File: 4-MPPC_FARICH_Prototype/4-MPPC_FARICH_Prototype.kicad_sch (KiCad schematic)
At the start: 33 parts, among them J1 1778764, J2 ST4-40-1.00-L-D-P-TR, J3 ST4-40-1.00-L-D-P-TR, J4 ST4-40-1.00-L-D-P-TR, J5 ST4-40-1.00-L-D-P-TR, J6 ST4-40-1.00-L-D-P-TR, J7 ST4-40-1.00-L-D-P-TR, J8 ST4-40-1.00-L-D-P-TR, J9 ST4-40-1.00-L-D-P-TR

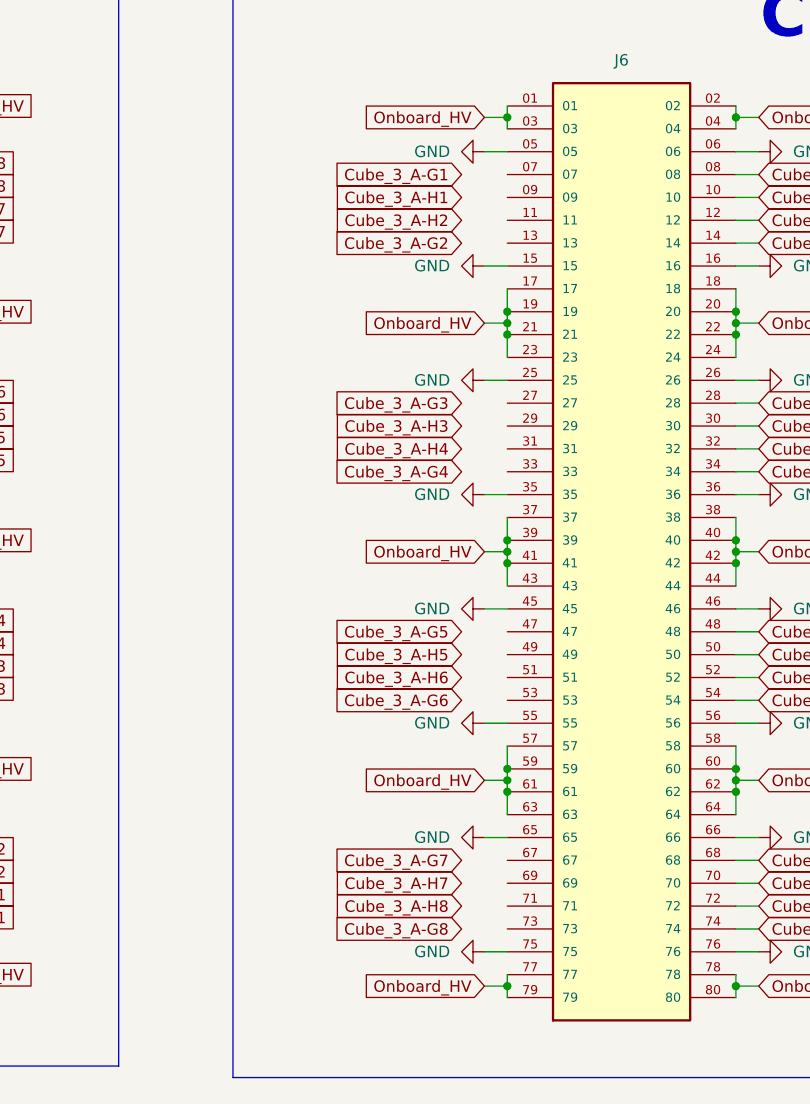
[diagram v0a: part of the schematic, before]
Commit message: .
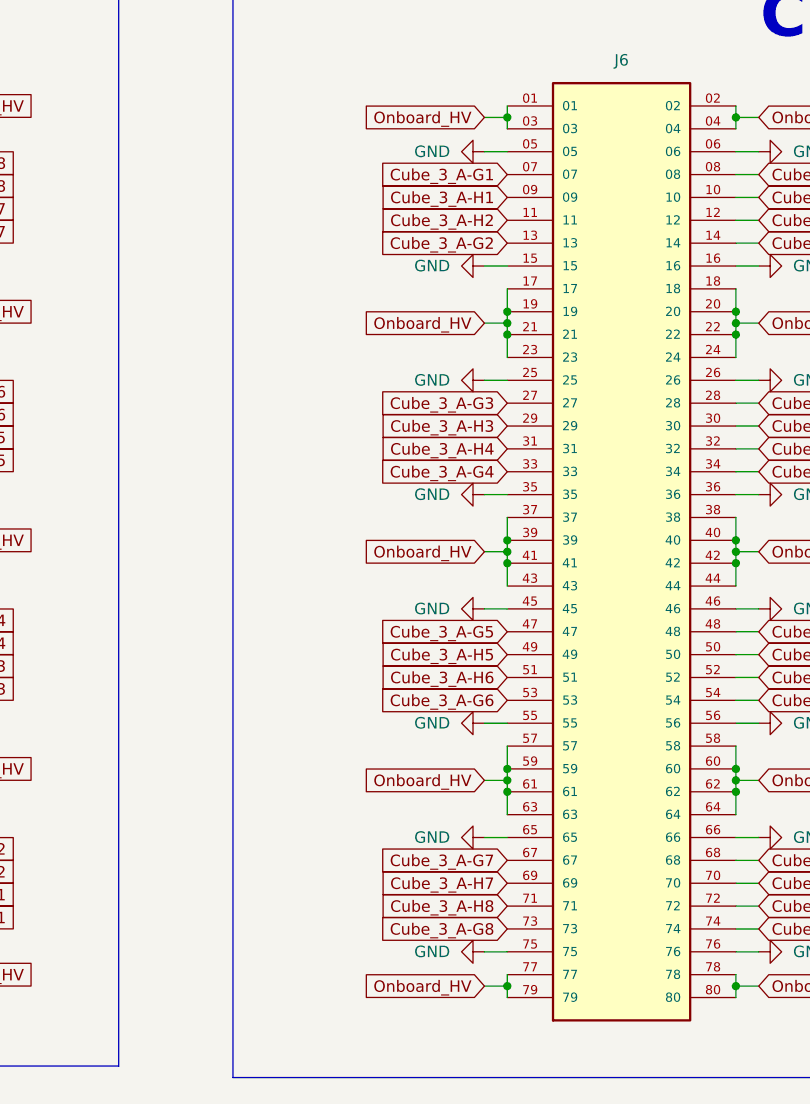
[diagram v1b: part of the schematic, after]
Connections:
- net Cube_3_A-G1: now also J6.07
- net Cube_3_A-G2: now also J6.13
- net Cube_3_A-G3: now also J6.27
- net Cube_3_A-G4: now also J6.33
- net Cube_3_A-G5: now also J6.47
- net Cube_3_A-G6: now also J6.53
- net Cube_3_A-G7: now also J6.67
- net Cube_3_A-G8: now also J6.73
- net Cube_3_A-H1: now also J6.09
- net Cube_3_A-H2: now also J6.11
- net Cube_3_A-H3: now also J6.29
- net Cube_3_A-H4: now also J6.31
- net Cube_3_A-H5: now also J6.49
- net Cube_3_A-H6: now also J6.51
- net Cube_3_A-H7: now also J6.69
- net Cube_3_A-H8: now also J6.71
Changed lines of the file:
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@@
 	(global_label "Cube_3_A-H4"
 		(shape input)
-		(at 232.41 320.04 180)
+		(at 237.49 320.04 180)
 		(fields_autoplaced yes)
 		(effects
@@
 		)
 		(property "Intersheetrefs" "${INTERSHEET_REFS}"
-			(at 216.4225 320.04 0)
+			(at 221.5025 320.04 0)
 			(effects
 				(font
@@
 	(global_label "Cube_3_A-H7"
 		(shape input)
-		(at 232.41 368.3 180)
+		(at 237.49 368.3 180)
 		(fields_autoplaced yes)
 		(effects
@@
 		)
 		(property "Intersheetrefs" "${INTERSHEET_REFS}"
-			(at 216.4225 368.3 0)
+			(at 221.5025 368.3 0)
 			(effects
 				(font
@@
 	(global_label "Cube_3_A-H8"
 		(shape input)
-		(at 232.41 370.84 180)
+		(at 237.49 370.84 180)
 		(fields_autoplaced yes)
 		(effects
@@
 		)
 		(property "Intersheetrefs" "${INTERSHEET_REFS}"
-			(at 216.4225 370.84 0)
+			(at 221.5025 370.84 0)
 			(effects
 				(font
@@
 	(global_label "Cube_3_A-H2"
 		(shape input)
-		(at 232.41 294.64 180)
+		(at 237.49 294.64 180)
 		(fields_autoplaced yes)
 		(effects
@@
 		)
 		(property "Intersheetrefs" "${INTERSHEET_REFS}"
-			(at 216.4225 294.64 0)
+			(at 221.5025 294.64 0)
 			(effects
 				(font
@@
 	(global_label "Cube_3_A-G7"
 		(shape input)
-		(at 232.41 365.76 180)
+		(at 237.49 365.76 180)
 		(fields_autoplaced yes)
 		(effects
@@
 		)
 		(property "Intersheetrefs" "${INTERSHEET_REFS}"
-			(at 216.483 365.76 0)
+			(at 221.563 365.76 0)
 			(effects
 				(font
@@
 	(global_label "Cube_3_A-H3"
 		(shape input)
-		(at 232.41 317.5 180)
+		(at 237.49 317.5 180)
 		(fields_autoplaced yes)
 		(effects
@@
 		)
 		(property "Intersheetrefs" "${INTERSHEET_REFS}"
-			(at 216.4225 317.5 0)
+			(at 221.5025 317.5 0)
 			(effects
 				(font
@@
 	(global_label "Cube_3_A-H5"
 		(shape input)
-		(at 232.41 342.9 180)
+		(at 237.49 342.9 180)
 		(fields_autoplaced yes)
 		(effects
@@
 		)
 		(property "Intersheetrefs" "${INTERSHEET_REFS}"
-			(at 216.4225 342.9 0)
+			(at 221.5025 342.9 0)
 			(effects
 				(font
@@
 	(global_label "Cube_3_A-G2"
 		(shape input)
-		(at 232.41 297.18 180)
+		(at 237.49 297.18 180)
 		(fields_autoplaced yes)
 		(effects
@@
 		)
 		(property "Intersheetrefs" "${INTERSHEET_REFS}"
-			(at 216.483 297.18 0)
+			(at 221.563 297.18 0)
 			(effects
 				(font
@@
 	(global_label "Cube_3_A-G6"
 		(shape input)
-		(at 232.41 347.98 180)
+		(at 237.49 347.98 180)
 		(fields_autoplaced yes)
 		(effects
@@
 		)
 		(property "Intersheetrefs" "${INTERSHEET_REFS}"
-			(at 216.483 347.98 0)
+			(at 221.563 347.98 0)
 			(effects
 				(font
@@
 	(global_label "Cube_3_A-G4"
 		(shape input)
-		(at 232.41 322.58 180)
+		(at 237.49 322.58 180)
 		(fields_autoplaced yes)
 		(effects
@@
 		)
 		(property "Intersheetrefs" "${INTERSHEET_REFS}"
-			(at 216.483 322.58 0)
+			(at 221.563 322.58 0)
 			(effects
 				(font
@@
 	(global_label "Cube_3_A-H6"
 		(shape input)
-		(at 232.41 345.44 180)
+		(at 237.49 345.44 180)
 		(fields_autoplaced yes)
 		(effects
@@
 		)
 		(property "Intersheetrefs" "${INTERSHEET_REFS}"
-			(at 216.4225 345.44 0)
+			(at 221.5025 345.44 0)
 			(effects
 				(font
@@
 	(global_label "Cube_3_A-H1"
 		(shape input)
-		(at 232.41 292.1 180)
+		(at 237.49 292.1 180)
 		(fields_autoplaced yes)
 		(effects
@@
 		)
 		(property "Intersheetrefs" "${INTERSHEET_REFS}"
-			(at 216.4225 292.1 0)
+			(at 221.5025 292.1 0)
 			(effects
 				(font
@@
 	(global_label "Cube_3_A-G3"
 		(shape input)
-		(at 232.41 314.96 180)
+		(at 237.49 314.96 180)
 		(fields_autoplaced yes)
 		(effects
@@
 		)
 		(property "Intersheetrefs" "${INTERSHEET_REFS}"
-			(at 216.483 314.96 0)
+			(at 221.563 314.96 0)
 			(effects
 				(font
@@
 	(global_label "Cube_3_A-G5"
 		(shape input)
-		(at 232.41 340.36 180)
+		(at 237.49 340.36 180)
 		(fields_autoplaced yes)
 		(effects
@@
 		)
 		(property "Intersheetrefs" "${INTERSHEET_REFS}"
-			(at 216.483 340.36 0)
+			(at 221.563 340.36 0)
 			(effects
 				(font
@@
 	(global_label "Cube_3_A-G1"
 		(shape input)
-		(at 232.41 289.56 180)
+		(at 237.49 289.56 180)
 		(fields_autoplaced yes)
 		(effects
@@
 		)
 		(property "Intersheetrefs" "${INTERSHEET_REFS}"
-			(at 216.483 289.56 0)
+			(at 221.563 289.56 0)
 			(effects
 				(font
@@
 	(global_label "Cube_3_A-G8"
 		(shape input)
-		(at 232.41 373.38 180)
+		(at 237.49 373.38 180)
 		(fields_autoplaced yes)
 		(effects
@@
 		)
 		(property "Intersheetrefs" "${INTERSHEET_REFS}"
-			(at 216.483 373.38 0)
+			(at 221.563 373.38 0)
 			(effects
 				(font
